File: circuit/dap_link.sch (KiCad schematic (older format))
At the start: 27 parts, among them J1 USB_A_CONN, J2 SWD_CONN_5P, J3 UART1_CONN_3P, U1 STM32F103CBTx, U2 AMS1117-3.3, Y1 8MHz

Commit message: 1
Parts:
- added J4: PAEX_CONN_6P, Connector_PinHeader_2.54mm:PinHeader_1x06_P2.54mm_Vertical, symbol Connector:Conn_01x06_Male
- added R11, R13, R14, R15, R16: 1K, Resistor_SMD:R_0603_1608Metric_Pad1.05x0.95mm_HandSolder, symbol Device:R
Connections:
- net labels added: PA0, PA1, PA2, PA3, PA4
- wire segments 92 -> 108
- no-connect marks 27 -> 22
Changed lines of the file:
@@
 Comment4 ""
 $EndDescr
-$Comp
-L MCU_ST_STM32F1:STM32F103CBTx U1
-U 1 1 5E71E086
-P 4450 3350
-F 0 "U1" H 4400 3300 50  0000 C CNN
-F 1 "STM32F103CBTx" H 4400 2800 50  0000 C CNN
-F 2 "Package_QFP:LQFP-48_7x7mm_P0.5mm" H 3850 1950 50  0001 R CNN
-F 3 "http://www.st.com/st-web-ui/static/active/en/resource/technical/document/datasheet/CD00161566.pdf" H 4450 3350 50  0001 C CNN
-	1    4450 3350
-	1    0    0    -1
-$EndComp
 Wire Wire Line
 	4350 1850 4350 1700
@@
 NoConn ~ 3750 2850
 NoConn ~ 3750 2750
-NoConn ~ 5050 3150
-NoConn ~ 5050 3250
-NoConn ~ 5050 3350
-NoConn ~ 5050 3450
-NoConn ~ 5050 3550
 NoConn ~ 5050 3650
 NoConn ~ 5050 3950
@@
 	1    0    0    -1
 $EndComp
+$Comp
+L MCU_ST_STM32F1:STM32F103CBTx U1
+U 1 1 5E71E086
+P 4450 3350
+F 0 "U1" H 4400 3300 50  0000 C CNN
+F 1 "STM32F103CBTx" H 4400 2800 50  0000 C CNN
+F 2 "Package_QFP:LQFP-48_7x7mm_P0.5mm" H 3850 1950 50  0001 R CNN
+F 3 "http://www.st.com/st-web-ui/static/active/en/resource/technical/document/datasheet/CD00161566.pdf" H 4450 3350 50  0001 C CNN
+	1    4450 3350
+	1    0    0    -1
+$EndComp
+Wire Wire Line
+	5050 3150 5400 3150
+Wire Wire Line
+	5050 3250 5400 3250
+Wire Wire Line
+	5050 3350 5400 3350
+Wire Wire Line
+	5050 3450 5400 3450
+Wire Wire Line
+	5050 3550 5400 3550
+Text Label 5250 3150 0    50   ~ 0
+PA0
+Text Label 5250 3250 0    50   ~ 0
+PA1
+Text Label 5250 3350 0    50   ~ 0
+PA2
+Text Label 5250 3450 0    50   ~ 0
+PA3
+Text Label 5250 3550 0    50   ~ 0
+PA4
+Wire Wire Line
+	4550 5550 4850 5550
+Wire Wire Line
+	4550 5650 4850 5650
+Wire Wire Line
+	4550 5750 4850 5750
+Wire Wire Line
+	4550 5850 4850 5850
+Wire Wire Line
+	4550 5950 4850 5950
+$Comp
+L Connector:Conn_01x06_Male J4
+U 1 1 5E7D84F3
+P 4350 5750
+F 0 "J4" H 4458 6131 50  0000 C CNN
+F 1 "PAEX_CONN_6P" H 4458 6040 50  0000 C CNN
+F 2 "Connector_PinHeader_2.54mm:PinHeader_1x06_P2.54mm_Vertical" H 4350 5750 50  0001 C CNN
+F 3 "~" H 4350 5750 50  0001 C CNN
+	1    4350 5750
+	1    0    0    -1
+$EndComp
+Wire Wire Line
+	4550 6050 4850 6050
+$Comp
+L power:GND #PWR06
+U 1 1 5E7DCB29
+P 4850 6050
+F 0 "#PWR06" H 4850 5800 50  0001 C CNN
+F 1 "GND" H 4855 5877 50  0000 C CNN
+F 2 "" H 4850 6050 50  0001 C CNN
+F 3 "" H 4850 6050 50  0001 C CNN
+	1    4850 6050
+	1    0    0    -1
+$EndComp
+Text Label 5250 5550 0    50   ~ 0
+PA0
+Text Label 5250 5650 0    50   ~ 0
+PA1
+Text Label 5250 5750 0    50   ~ 0
+PA2
+Text Label 5250 5850 0    50   ~ 0
+PA3
+Text Label 5250 5950 0    50   ~ 0
+PA4
+$Comp
+L Device:R R11
+U 1 1 5E79F696
+P 5000 5550
+F 0 "R11" V 4950 5400 50  0000 C CNN
+F 1 "1K" V 4950 5700 50  0000 C CNN
+F 2 "Resistor_SMD:R_0603_1608Metric_Pad1.05x0.95mm_HandSolder" V 4930 5550 50  0001 C CNN
+F 3 "~" H 5000 5550 50  0001 C CNN
+	1    5000 5550
+	0    1    1    0
+$EndComp
+$Comp
+L Device:R R13
+U 1 1 5E79FF83
+P 5000 5650
+F 0 "R13" V 4950 5500 50  0000 C CNN
+F 1 "1K" V 4950 5800 50  0000 C CNN
+F 2 "Resistor_SMD:R_0603_1608Metric_Pad1.05x0.95mm_HandSolder" V 4930 5650 50  0001 C CNN
+F 3 "~" H 5000 5650 50  0001 C CNN
+	1    5000 5650
+	0    1    1    0
+$EndComp
+$Comp
+L Device:R R14
+U 1 1 5E7A0232
+P 5000 5750
+F 0 "R14" V 4950 5600 50  0000 C CNN
+F 1 "1K" V 4950 5900 50  0000 C CNN
+F 2 "Resistor_SMD:R_0603_1608Metric_Pad1.05x0.95mm_HandSolder" V 4930 5750 50  0001 C CNN
+F 3 "~" H 5000 5750 50  0001 C CNN
+	1    5000 5750
+	0    1    1    0
+$EndComp
+$Comp
+L Device:R R15
+U 1 1 5E7A0411
+P 5000 5850
+F 0 "R15" V 4950 5700 50  0000 C CNN
+F 1 "1K" V 4950 6000 50  0000 C CNN
+F 2 "Resistor_SMD:R_0603_1608Metric_Pad1.05x0.95mm_HandSolder" V 4930 5850 50  0001 C CNN
+F 3 "~" H 5000 5850 50  0001 C CNN
+	1    5000 5850
+	0    1    1    0
+$EndComp
+$Comp
+L Device:R R16
+U 1 1 5E7A06A9
+P 5000 5950
+F 0 "R16" V 4950 5800 50  0000 C CNN
+F 1 "1K" V 4950 6100 50  0000 C CNN
+F 2 "Resistor_SMD:R_0603_1608Metric_Pad1.05x0.95mm_HandSolder" V 4930 5950 50  0001 C CNN
+F 3 "~" H 5000 5950 50  0001 C CNN
+	1    5000 5950
+	0    1    1    0
+$EndComp
+Wire Wire Line
+	5150 5550 5300 5550
+Wire Wire Line
+	5150 5650 5300 5650
+Wire Wire Line
+	5150 5750 5300 5750
+Wire Wire Line
+	5150 5850 5300 5850
+Wire Wire Line
+	5150 5950 5300 5950
 $EndSCHEMATC

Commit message: DA111
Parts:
- added R17, R18: 1K, Resistor_SMD:R_0603_1608Metric_Pad1.05x0.95mm_HandSolder, symbol Device:R
- J4: value PAEX_CONN_6P -> PAEX_CONN_8P; footprint Connector_PinHeader_2.54mm:PinHeader_1x06_P2.54mm_Vertical -> Connector_PinHeader_2.54mm:PinHeader_1x08_P2.54mm_Vertical; symbol Connector:Conn_01x06_Male -> Connector:Conn_01x08_Male
- U1: symbol MCU_ST_STM32F1:STM32F103CBTx -> dap_link-rescue:STM32F103CBTx-MCU_ST_STM32F1
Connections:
- net labels added: PA5, PA6
- wire segments 108 -> 114
- no-connect marks 22 -> 20
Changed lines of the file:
@@
 U 1 1 5E77CF74
 P 5700 4050
-F 0 "R6" V 5600 3950 50  0000 C CNN
-F 1 "100R" V 5600 4150 50  0000 C CNN
+F 0 "R6" V 5650 3900 50  0000 C CNN
+F 1 "100R" V 5650 4250 50  0000 C CNN
 F 2 "Resistor_SMD:R_0603_1608Metric_Pad1.05x0.95mm_HandSolder" V 5630 4050 50  0001 C CNN
 F 3 "~" H 5700 4050 50  0001 C CNN
@@
 U 1 1 5E77D476
 P 5700 4150
-F 0 "R7" V 5800 4100 50  0000 C CNN
-F 1 "100R" V 5800 4300 50  0000 C CNN
+F 0 "R7" V 5650 4000 50  0000 C CNN
+F 1 "100R" V 5650 4350 50  0000 C CNN
 F 2 "Resistor_SMD:R_0603_1608Metric_Pad1.05x0.95mm_HandSolder" V 5630 4150 50  0001 C CNN
 F 3 "~" H 5700 4150 50  0001 C CNN
@@
 SWCLK
 Wire Wire Line
-	5050 3750 5600 3750
-Wire Wire Line
 	5050 3850 5600 3850
-Text Label 5350 3750 0    50   ~ 0
+Wire Wire Line
+	5050 3950 5600 3950
+Text Label 5350 3850 0    50   ~ 0
 LEDR_GPIO
-Text Label 5350 3850 0    50   ~ 0
+Text Label 5350 3950 0    50   ~ 0
 LEDG_GPIO
 $Comp
@@
 NoConn ~ 3750 2850
 NoConn ~ 3750 2750
-NoConn ~ 5050 3650
-NoConn ~ 5050 3950
-$Comp
-L power:GND_USB #PWR0101
+$Comp
+L dap_link-rescue:GND_USB-power #PWR0101
 U 1 1 5E860E4C
 P 8500 2450
@@
 	8500 2350 8500 2450
 $Comp
-L power:VCC_USB #PWR0102
+L dap_link-rescue:VCC_USB-power #PWR0102
 U 1 1 5E787AD2
 P 9050 1350
@@
 $EndComp
 $Comp
-L power:VCC_USB #PWR0103
+L dap_link-rescue:VCC_USB-power #PWR0103
 U 1 1 5E78A027
 P 7550 3700
@@
 $EndComp
 $Comp
-L MCU_ST_STM32F1:STM32F103CBTx U1
+L dap_link-rescue:STM32F103CBTx-MCU_ST_STM32F1 U1
 U 1 1 5E71E086
 P 4450 3350
@@
 	4550 5950 4850 5950
 $Comp
-L Connector:Conn_01x06_Male J4
+L Connector:Conn_01x08_Male J4
 U 1 1 5E7D84F3
-P 4350 5750
-F 0 "J4" H 4458 6131 50  0000 C CNN
-F 1 "PAEX_CONN_6P" H 4458 6040 50  0000 C CNN
-F 2 "Connector_PinHeader_2.54mm:PinHeader_1x06_P2.54mm_Vertical" H 4350 5750 50  0001 C CNN
-F 3 "~" H 4350 5750 50  0001 C CNN
-	1    4350 5750
-	1    0    0    -1
-$EndComp
-Wire Wire Line
-	4550 6050 4850 6050
+P 4350 5850
+F 0 "J4" H 4350 6250 50  0000 C CNN
+F 1 "PAEX_CONN_8P" H 4300 5350 50  0000 C CNN
+F 2 "Connector_PinHeader_2.54mm:PinHeader_1x08_P2.54mm_Vertical" H 4350 5850 50  0001 C CNN
+F 3 "~" H 4350 5850 50  0001 C CNN
+	1    4350 5850
+	1    0    0    -1
+$EndComp
+Wire Wire Line
+	4550 6250 4850 6250
 $Comp
 L power:GND #PWR06
 U 1 1 5E7DCB29
-P 4850 6050
-F 0 "#PWR06" H 4850 5800 50  0001 C CNN
-F 1 "GND" H 4855 5877 50  0000 C CNN
-F 2 "" H 4850 6050 50  0001 C CNN
-F 3 "" H 4850 6050 50  0001 C CNN
-	1    4850 6050
+P 4850 6250
+F 0 "#PWR06" H 4850 6000 50  0001 C CNN
+F 1 "GND" H 4855 6077 50  0000 C CNN
+F 2 "" H 4850 6250 50  0001 C CNN
+F 3 "" H 4850 6250 50  0001 C CNN
+	1    4850 6250
 	1    0    0    -1
 $EndComp
@@
 U 1 1 5E79F696
 P 5000 5550
-F 0 "R11" V 4950 5400 50  0000 C CNN
+F 0 "R11" V 4950 5350 50  0000 C CNN
 F 1 "1K" V 4950 5700 50  0000 C CNN
 F 2 "Resistor_SMD:R_0603_1608Metric_Pad1.05x0.95mm_HandSolder" V 4930 5550 50  0001 C CNN
@@
 U 1 1 5E79FF83
 P 5000 5650
-F 0 "R13" V 4950 5500 50  0000 C CNN
+F 0 "R13" V 4950 5450 50  0000 C CNN
 F 1 "1K" V 4950 5800 50  0000 C CNN
 F 2 "Resistor_SMD:R_0603_1608Metric_Pad1.05x0.95mm_HandSolder" V 4930 5650 50  0001 C CNN
@@
 U 1 1 5E7A0232
 P 5000 5750
-F 0 "R14" V 4950 5600 50  0000 C CNN
+F 0 "R14" V 4950 5550 50  0000 C CNN
 F 1 "1K" V 4950 5900 50  0000 C CNN
 F 2 "Resistor_SMD:R_0603_1608Metric_Pad1.05x0.95mm_HandSolder" V 4930 5750 50  0001 C CNN
@@
 U 1 1 5E7A0411
 P 5000 5850
-F 0 "R15" V 4950 5700 50  0000 C CNN
+F 0 "R15" V 4950 5650 50  0000 C CNN
 F 1 "1K" V 4950 6000 50  0000 C CNN
 F 2 "Resistor_SMD:R_0603_1608Metric_Pad1.05x0.95mm_HandSolder" V 4930 5850 50  0001 C CNN
@@
 U 1 1 5E7A06A9
 P 5000 5950
-F 0 "R16" V 4950 5800 50  0000 C CNN
+F 0 "R16" V 4950 5750 50  0000 C CNN
 F 1 "1K" V 4950 6100 50  0000 C CNN
 F 2 "Resistor_SMD:R_0603_1608Metric_Pad1.05x0.95mm_HandSolder" V 4930 5950 50  0001 C CNN
@@
 Wire Wire Line
 	5150 5950 5300 5950
+Wire Wire Line
+	5050 3650 5400 3650
+Wire Wire Line
+	5050 3750 5400 3750
+Text Label 5250 3650 0    50   ~ 0
+PA5
+Text Label 5250 3750 0    50   ~ 0
+PA6
+$Comp
+L Device:R R17
+U 1 1 5E7D1F62
+P 5000 6050
+F 0 "R17" V 4950 5850 50  0000 C CNN
+F 1 "1K" V 4950 6200 50  0000 C CNN
+F 2 "Resistor_SMD:R_0603_1608Metric_Pad1.05x0.95mm_HandSolder" V 4930 6050 50  0001 C CNN
+F 3 "~" H 5000 6050 50  0001 C CNN
+	1    5000 6050
+	0    1    1    0
+$EndComp
+$Comp
+L Device:R R18
+U 1 1 5E7D20D9
+P 5000 6150
+F 0 "R18" V 4950 5950 50  0000 C CNN
+F 1 "1K" V 4950 6300 50  0000 C CNN
+F 2 "Resistor_SMD:R_0603_1608Metric_Pad1.05x0.95mm_HandSolder" V 4930 6150 50  0001 C CNN
+F 3 "~" H 5000 6150 50  0001 C CNN
+	1    5000 6150
+	0    1    1    0
+$EndComp
+Wire Wire Line
+	4550 6050 4850 6050
+Wire Wire Line
+	4550 6150 4850 6150
+Wire Wire Line
+	5150 6050 5300 6050
+Wire Wire Line
+	5150 6150 5300 6150
+Text Label 5250 6050 0    50   ~ 0
+PA5
+Text Label 5250 6150 0    50   ~ 0
+PA6
 $EndSCHEMATC

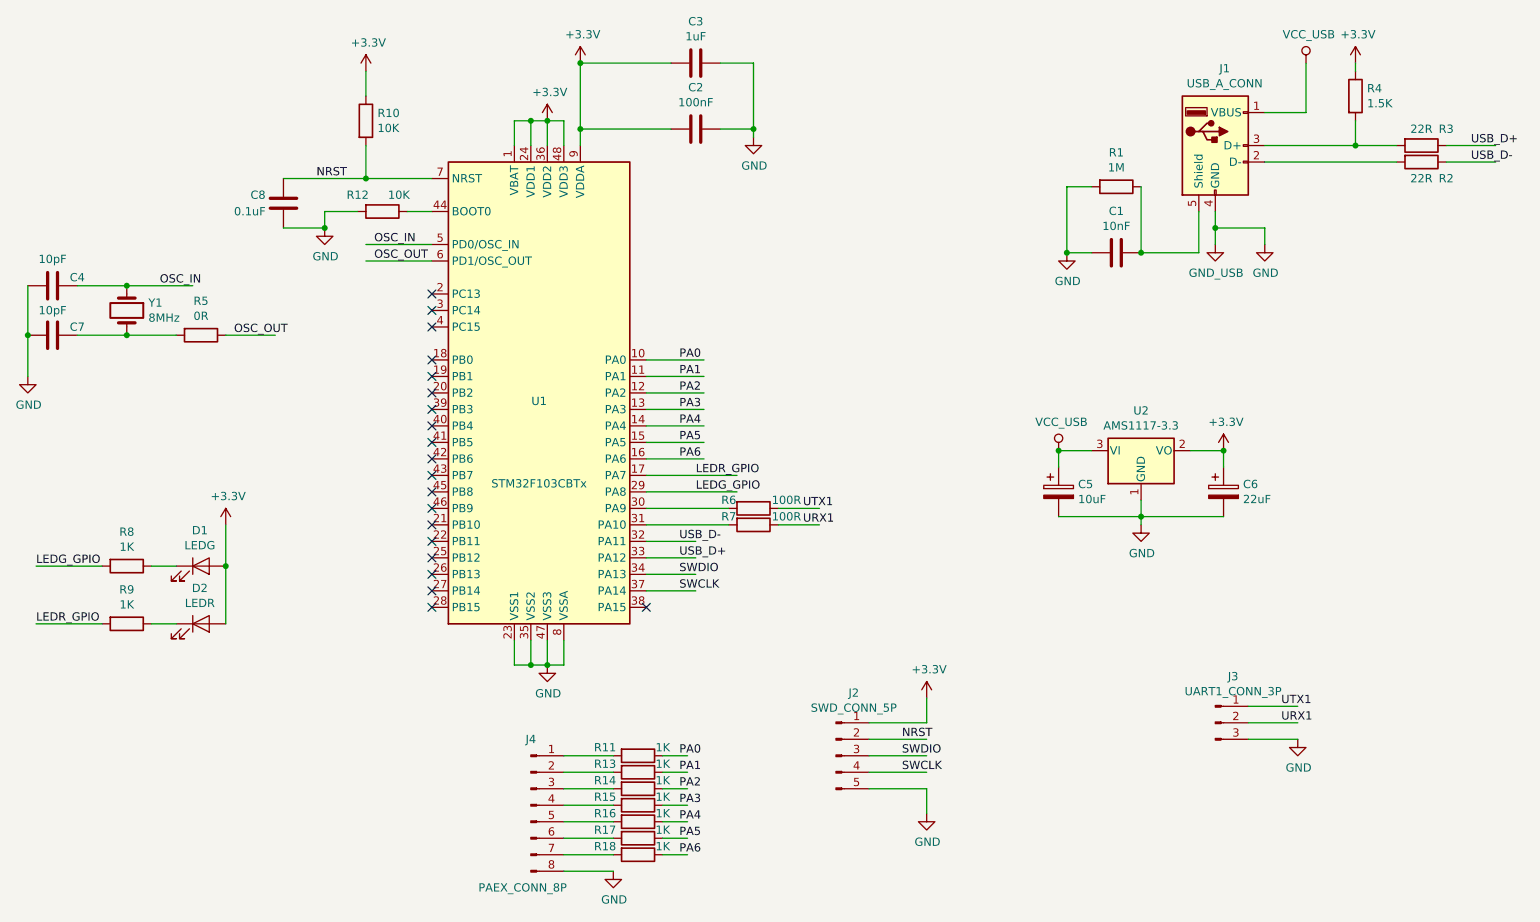
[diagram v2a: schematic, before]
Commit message: 1
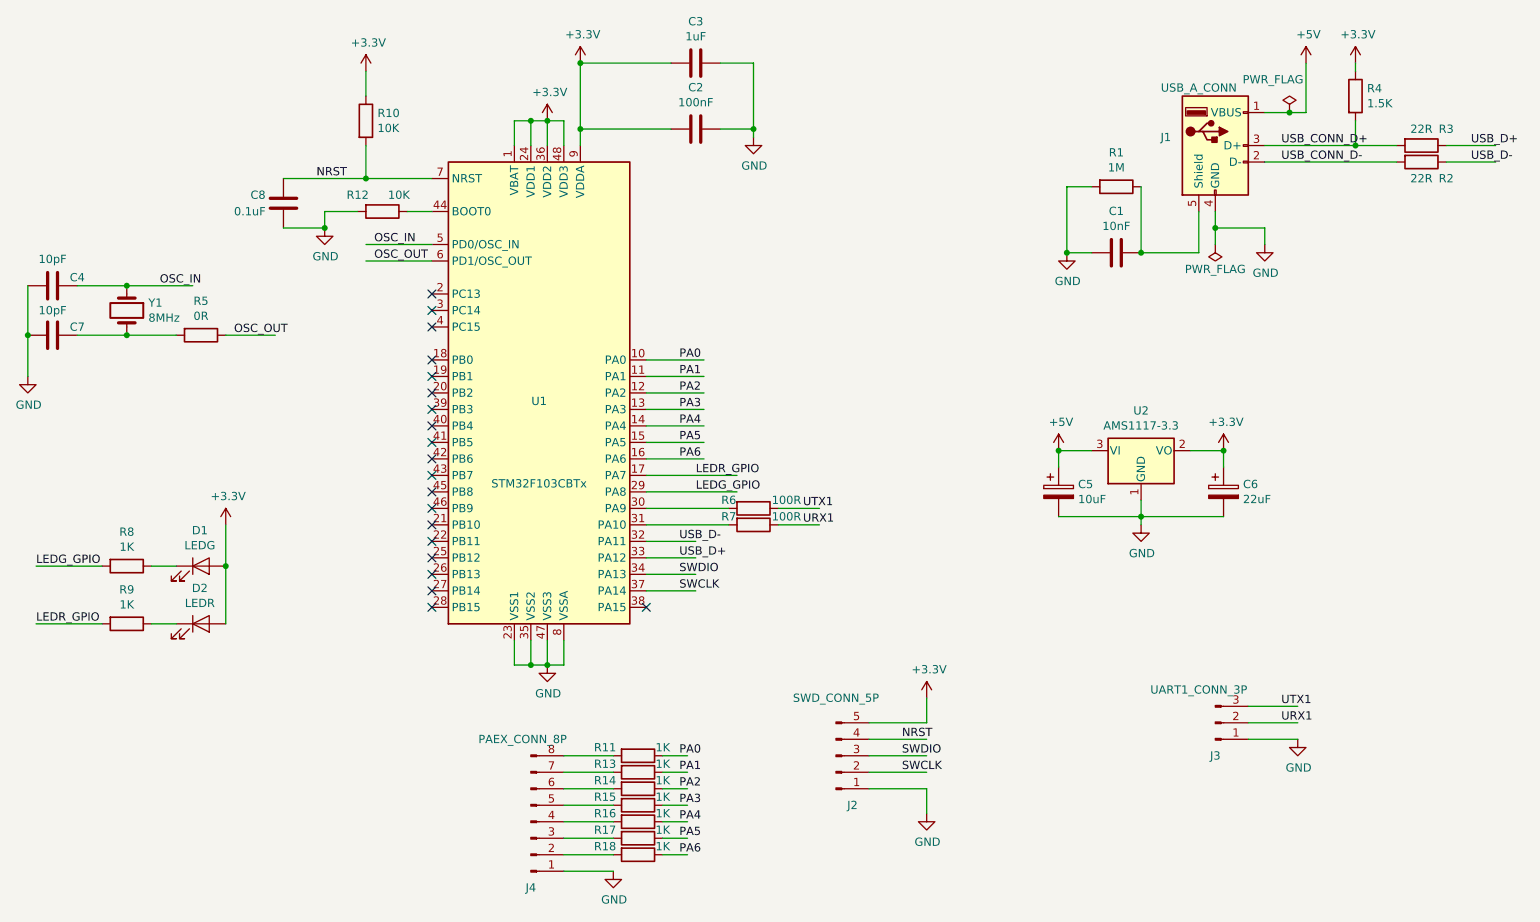
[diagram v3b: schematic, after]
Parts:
- J4: footprint Connector_PinHeader_2.54mm:PinHeader_1x08_P2.54mm_Vertical -> Connector_PinHeader_2.54mm:PinHeader_1x08_P2.54mm_Horizontal
- Y1: footprint Crystal:Crystal_SMD_SeikoEpson_MA505-2Pin_12.7x5.1mm -> Crystal:Crystal_SMD_SeikoEpson_MC405-2Pin_9.6x4.1mm
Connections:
- net labels added: +5V, USB_CONN_D+, USB_CONN_D-
- net labels removed: GND_USB, VCC_USB
- wire segments 114 -> 115
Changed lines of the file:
@@
 U 1 1 5E760A0A
 P 8500 1850
-F 0 "J1" H 8557 2317 50  0000 C CNN
-F 1 "USB_A_CONN" H 8557 2226 50  0000 C CNN
+F 0 "J1" H 8200 1900 50  0000 C CNN
+F 1 "USB_A_CONN" H 8400 2200 50  0000 C CNN
 F 2 "Connector_USB:USB_A_CNCTech_1001-011-01101_Horizontal" H 8650 1800 50  0001 C CNN
 F 3 " ~" H 8650 1800 50  0001 C CNN
@@
 $EndComp
 Wire Wire Line
-	8800 1650 9050 1650
+	8800 1650 8950 1650
 Text Label 10050 1850 0    50   ~ 0
 USB_D+
@@
 F 0 "Y1" V 1854 2981 50  0000 L CNN
 F 1 "8MHz" V 1945 2981 50  0000 L CNN
-F 2 "Crystal:Crystal_SMD_SeikoEpson_MA505-2Pin_12.7x5.1mm" H 1900 2850 50  0001 C CNN
+F 2 "Crystal:Crystal_SMD_SeikoEpson_MC405-2Pin_9.6x4.1mm" H 1900 2850 50  0001 C CNN
 F 3 "~" H 1900 2850 50  0001 C CNN
 	1    1900 2850
@@
 U 1 1 5E78FA1B
 P 8500 5350
-F 0 "J3" H 8608 5631 50  0000 C CNN
-F 1 "UART1_CONN_3P" H 8608 5540 50  0000 C CNN
+F 0 "J3" H 8500 5550 50  0000 C CNN
+F 1 "UART1_CONN_3P" H 8400 5150 50  0000 C CNN
 F 2 "Connector_PinHeader_2.54mm:PinHeader_1x03_P2.54mm_Vertical" H 8500 5350 50  0001 C CNN
 F 3 "~" H 8500 5350 50  0001 C CNN
 	1    8500 5350
-	1    0    0    -1
+	1    0    0    1
 $EndComp
 Wire Wire Line
@@
 U 1 1 5E7B3ABB
 P 6200 5550
-F 0 "J2" H 6308 5931 50  0000 C CNN
-F 1 "SWD_CONN_5P" H 6308 5840 50  0000 C CNN
+F 0 "J2" H 6300 5850 50  0000 C CNN
+F 1 "SWD_CONN_5P" H 6200 5200 50  0000 C CNN
 F 2 "Connector_PinHeader_2.54mm:PinHeader_1x05_P2.54mm_Vertical" H 6200 5550 50  0001 C CNN
 F 3 "~" H 6200 5550 50  0001 C CNN
 	1    6200 5550
-	1    0    0    -1
+	1    0    0    1
 $EndComp
 Wire Wire Line
@@
 NoConn ~ 3750 2850
 NoConn ~ 3750 2750
-$Comp
-L dap_link-rescue:GND_USB-power #PWR0101
-U 1 1 5E860E4C
-P 8500 2450
-F 0 "#PWR0101" H 8500 2200 50  0001 C CNN
-F 1 "GND_USB" H 8505 2277 50  0000 C CNN
-F 2 "" H 8500 2450 50  0001 C CNN
-F 3 "" H 8500 2450 50  0001 C CNN
-	1    8500 2450
-	1    0    0    -1
-$EndComp
 Wire Wire Line
 	8500 2350 8800 2350
@@
 Wire Wire Line
 	8500 2350 8500 2450
-$Comp
-L dap_link-rescue:VCC_USB-power #PWR0102
-U 1 1 5E787AD2
-P 9050 1350
-F 0 "#PWR0102" H 9200 1300 50  0001 C CNN
-F 1 "VCC_USB" H 9067 1523 50  0000 C CNN
-F 2 "" H 9050 1350 50  0001 C CNN
-F 3 "" H 9050 1350 50  0001 C CNN
-	1    9050 1350
-	1    0    0    -1
-$EndComp
-$Comp
-L dap_link-rescue:VCC_USB-power #PWR0103
-U 1 1 5E78A027
-P 7550 3700
-F 0 "#PWR0103" H 7700 3650 50  0001 C CNN
-F 1 "VCC_USB" H 7567 3873 50  0000 C CNN
-F 2 "" H 7550 3700 50  0001 C CNN
-F 3 "" H 7550 3700 50  0001 C CNN
-	1    7550 3700
-	1    0    0    -1
-$EndComp
-Connection ~ 7550 3700
 $Comp
 L power:GND #PWR0104
@@
 L Connector:Conn_01x08_Male J4
 U 1 1 5E7D84F3
-P 4350 5850
-F 0 "J4" H 4350 6250 50  0000 C CNN
-F 1 "PAEX_CONN_8P" H 4300 5350 50  0000 C CNN
-F 2 "Connector_PinHeader_2.54mm:PinHeader_1x08_P2.54mm_Vertical" H 4350 5850 50  0001 C CNN
-F 3 "~" H 4350 5850 50  0001 C CNN
-	1    4350 5850
-	1    0    0    -1
+P 4350 5950
+F 0 "J4" H 4350 6350 50  0000 C CNN
+F 1 "PAEX_CONN_8P" H 4300 5450 50  0000 C CNN
+F 2 "Connector_PinHeader_2.54mm:PinHeader_1x08_P2.54mm_Horizontal" H 4350 5950 50  0001 C CNN
+F 3 "~" H 4350 5950 50  0001 C CNN
+	1    4350 5950
+	1    0    0    1
 $EndComp
 Wire Wire Line
@@
 Text Label 5250 6150 0    50   ~ 0
 PA6
+$Comp
+L power:+5V #PWR0101
+U 1 1 5E8C47C9
+P 9050 1350
+F 0 "#PWR0101" H 9050 1200 50  0001 C CNN
+F 1 "+5V" H 9065 1523 50  0000 C CNN
+F 2 "" H 9050 1350 50  0001 C CNN
+F 3 "" H 9050 1350 50  0001 C CNN
+	1    9050 1350
+	1    0    0    -1
+$EndComp
+$Comp
+L power:+5V #PWR0102
+U 1 1 5E8C5485
+P 7550 3700
+F 0 "#PWR0102" H 7550 3550 50  0001 C CNN
+F 1 "+5V" H 7565 3873 50  0000 C CNN
+F 2 "" H 7550 3700 50  0001 C CNN
+F 3 "" H 7550 3700 50  0001 C CNN
+	1    7550 3700
+	1    0    0    -1
+$EndComp
+Connection ~ 7550 3700
+$Comp
+L power:PWR_FLAG #FLG0101
+U 1 1 5E8CAC71
+P 8950 1650
+F 0 "#FLG0101" H 8950 1725 50  0001 C CNN
+F 1 "PWR_FLAG" H 8850 1850 50  0000 C CNN
+F 2 "" H 8950 1650 50  0001 C CNN
+F 3 "~" H 8950 1650 50  0001 C CNN
+	1    8950 1650
+	1    0    0    -1
+$EndComp
+Connection ~ 8950 1650
+Wire Wire Line
+	8950 1650 9050 1650
+$Comp
+L power:PWR_FLAG #FLG0102
+U 1 1 5E8CC3CB
+P 8500 2450
+F 0 "#FLG0102" H 8500 2525 50  0001 C CNN
+F 1 "PWR_FLAG" H 8500 2600 50  0000 C CNN
+F 2 "" H 8500 2450 50  0001 C CNN
+F 3 "~" H 8500 2450 50  0001 C CNN
+	1    8500 2450
+	-1   0    0    1
+$EndComp
+Text Label 8900 1850 0    50   ~ 0
+USB_CONN_D+
+Text Label 8900 1950 0    50   ~ 0
+USB_CONN_D-
 $EndSCHEMATC

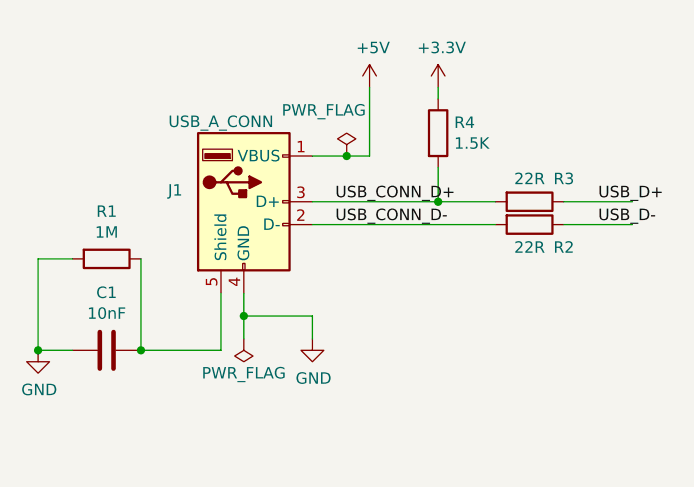
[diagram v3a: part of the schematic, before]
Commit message: 1333
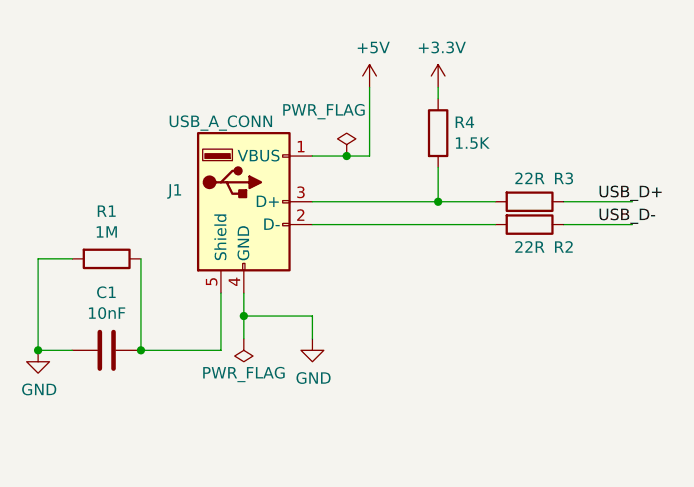
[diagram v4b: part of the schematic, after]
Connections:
- net labels removed: USB_CONN_D+, USB_CONN_D-
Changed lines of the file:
@@
 Wire Wire Line
 	8800 1650 8950 1650
-Text Label 10050 1850 0    50   ~ 0
-USB_D+
-Text Label 10050 1950 0    50   ~ 0
-USB_D-
 Wire Wire Line
 	8500 2250 8500 2350
@@
 	-1   0    0    1
 $EndComp
-Text Label 8900 1850 0    50   ~ 0
-USB_CONN_D+
-Text Label 8900 1950 0    50   ~ 0
-USB_CONN_D-
+Text Label 10050 1950 0    50   ~ 0
+USB_D-
+Text Label 10050 1850 0    50   ~ 0
+USB_D+
 $EndSCHEMATC
